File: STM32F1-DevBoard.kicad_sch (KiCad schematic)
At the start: 32 parts, among them SW1 SW_Push, SW2 SW_Push, U1 STM32F103C8T6, U2 AMS1117-3.3, U3 W25Q32JVSS

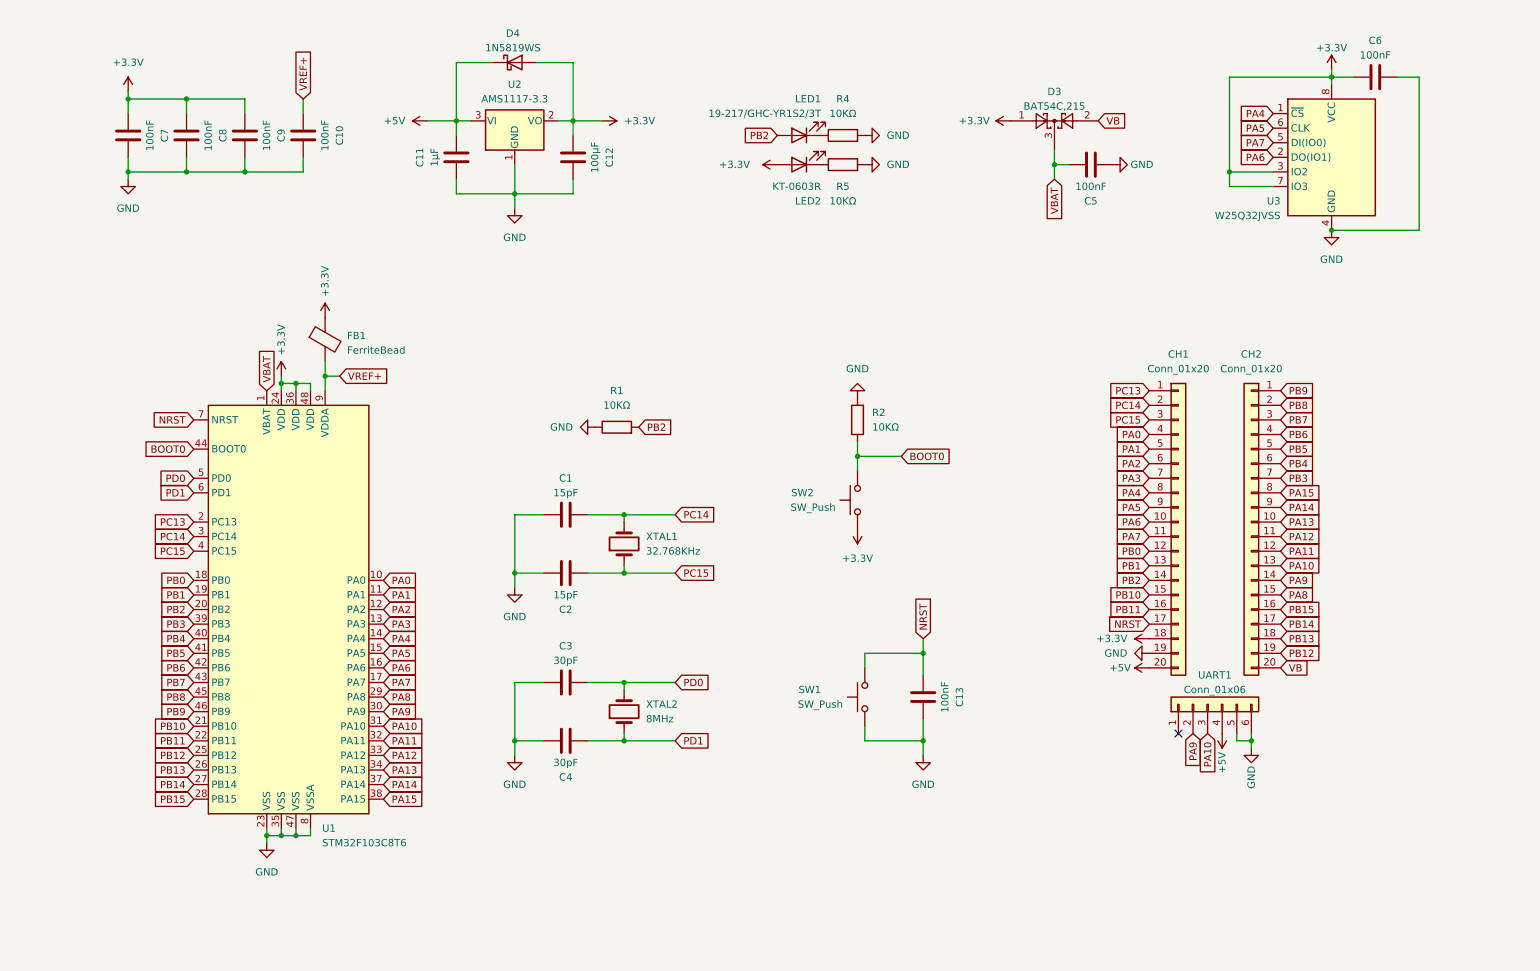
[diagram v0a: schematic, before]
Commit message: Add files via upload
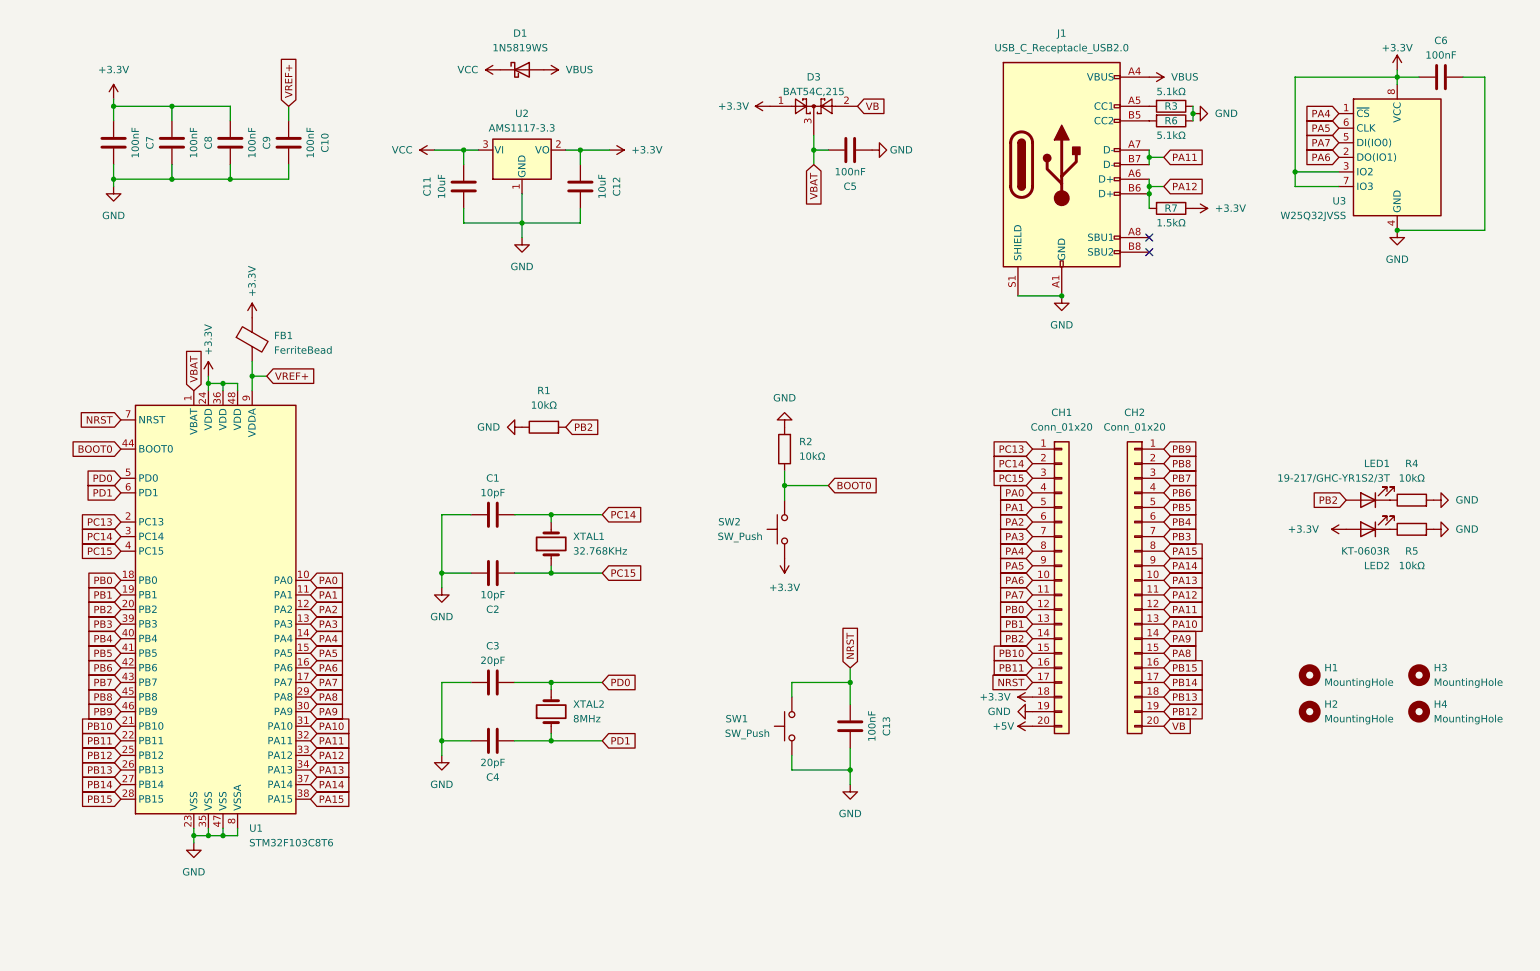
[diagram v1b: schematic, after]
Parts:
- removed D4: 1N5819WS, Diode_SMD:D_SOD-323, symbol Diode:1N5819WS
- removed UART1: Conn_01x06, Connector_PinHeader_2.54mm:PinHeader_1x06_P2.54mm_Horizontal, symbol Connector_Generic:Conn_01x06
- added D1: 1N5819WS, Diode_SMD:D_SOD-323, symbol Diode:1N5819WS
- added H1, H2, H3, H4: MountingHole, MountingHole:MountingHole_2.2mm_M2, symbol Mechanical:MountingHole
- added J1: USB_C_Receptacle_USB2.0, Connector_USB:USB_C_Receptacle_XKB_U262-16XN-4BVC11, symbol Connector:USB_C_Receptacle_USB2.0
- added R3, R6: 5.1kΩ, Resistor_SMD:R_0402_1005Metric, symbol Device:R
- added R7: 1.5kΩ, Resistor_SMD:R_0402_1005Metric, symbol Device:R
- C1, C2: value 15pF -> 10pF; LCSC C1548 -> C32949
- C11: value 1μF -> 10uF; LCSC C52923 -> C15525
- C12: value 100μF -> 10uF; footprint Capacitor_SMD:C_1206_3216Metric -> Capacitor_SMD:C_0402_1005Metric; LCSC C15008 -> C15525
- C3, C4: value 30pF -> 20pF; LCSC C1570 -> C1554
- C6: footprint Capacitor_SMD:C_0603_1608Metric -> Capacitor_SMD:C_0603_1608Metric_Pad1.08x0.95mm_HandSolder; LCSC (none) -> C14663
- R1, R2, R4, R5: value 10KΩ -> 10kΩ
- XTAL2: footprint Crystal:Crystal_SMD_HC49-SD -> Crystal:Crystal_SMD_5032-2Pin_5.0x3.2mm; LCSC C12674 -> C115962
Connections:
- net +3.3V: now also R7.1
- net +5V: no longer C11.1, U2.3 (VI)
- net GND: now also C2.2, C4.2, J1.A1 (GND), J1.A12 (GND), J1.B1 (GND), J1.B12 (GND), J1.S1 (SHIELD), R3.1, R6.1; no longer C2.1, C4.1
- net PA11: now also J1.A7 (D-), J1.B7 (D-)
- net PA12: now also J1.A6 (D+), J1.B6 (D+), R7.2
- net PC15: now also C2.1; no longer C2.2
- net PD1: now also C4.1; no longer C4.2
- new net: J1.B5 (CC2), R6.2
- new net: J1.A5 (CC1), R3.2
- new net VBUS: D1.2 (A), J1.A4 (VBUS), J1.A9 (VBUS), J1.B4 (VBUS), J1.B9 (VBUS)
- new net VCC: C11.1, D1.1 (K), U2.3 (VI)
- no-connect marks 1 -> 2
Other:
- title: STM32F103C8T6 -> STM32F1-DevBoard
- moved on the sheet: C1, C10, C11, C12, C13, C3, C5, C6, C7, C8, C9, CH1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

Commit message: Add files via upload
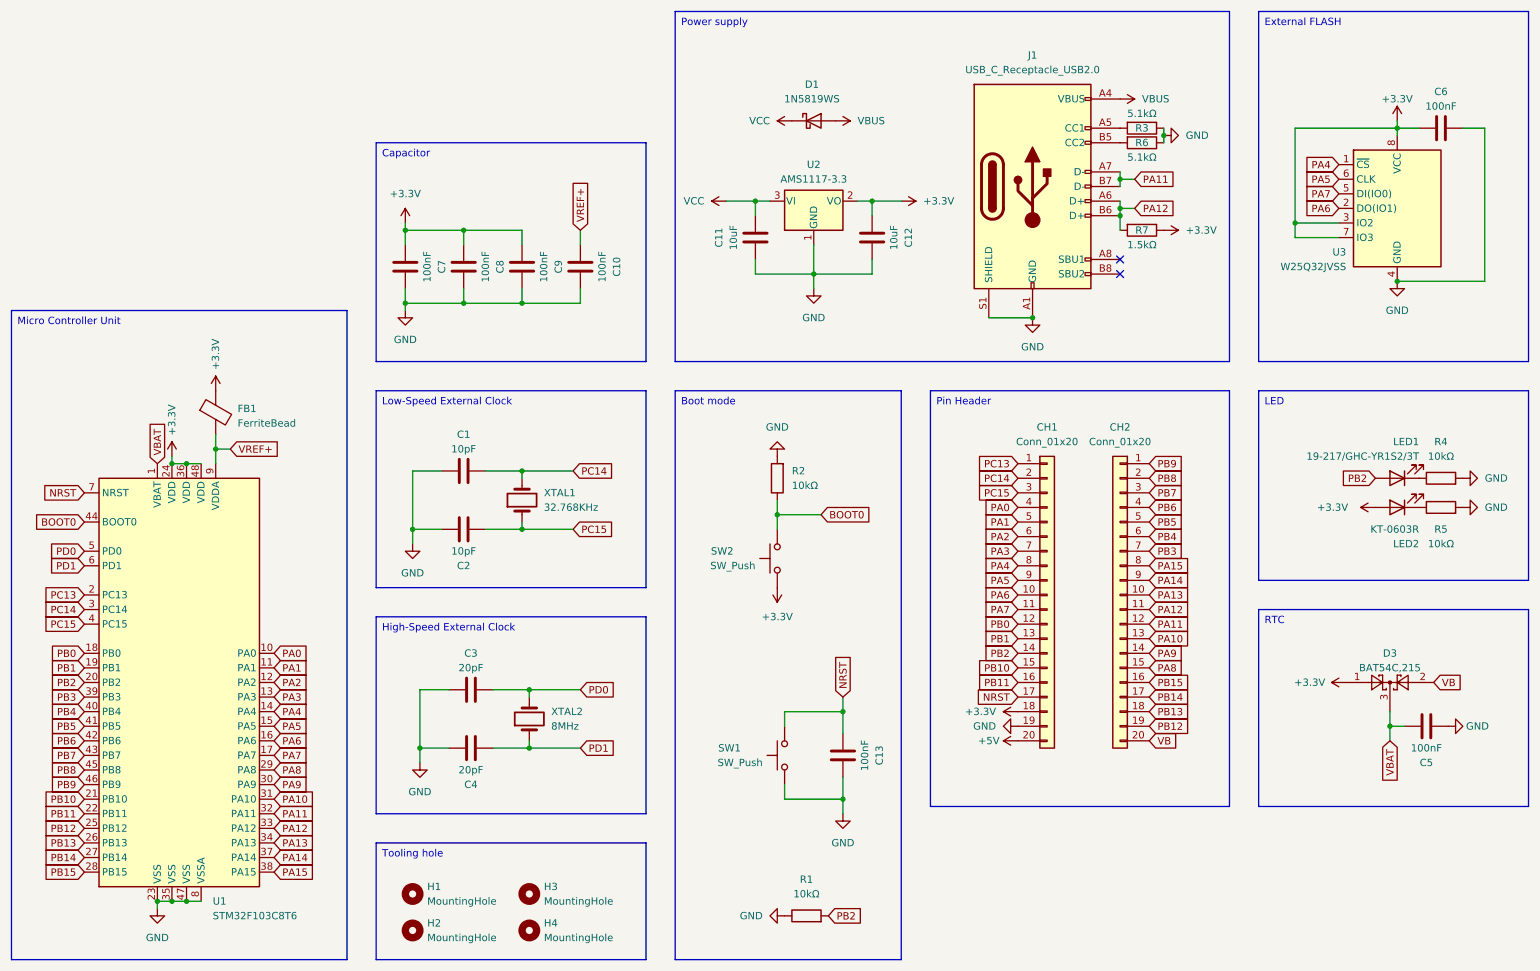
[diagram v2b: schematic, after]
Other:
- moved on the sheet: C1, C10, C11, C12, C13, C2, C3, C4, C5, C6, C7, C8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
